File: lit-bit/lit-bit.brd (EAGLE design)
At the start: 37.5 x 43.8 mm, 71 parts, among them J2 USB_MICRO_B_SMD_FEMALE, J3 ISP, U2 32U4, U3 73831, U4 ADXL345, U5 S-1335, U6 MCP7940N, U7 24FC1025, Y1 8MHz, Y2 32.768kHz, Y3 32.768kHz, Y4 16MHz

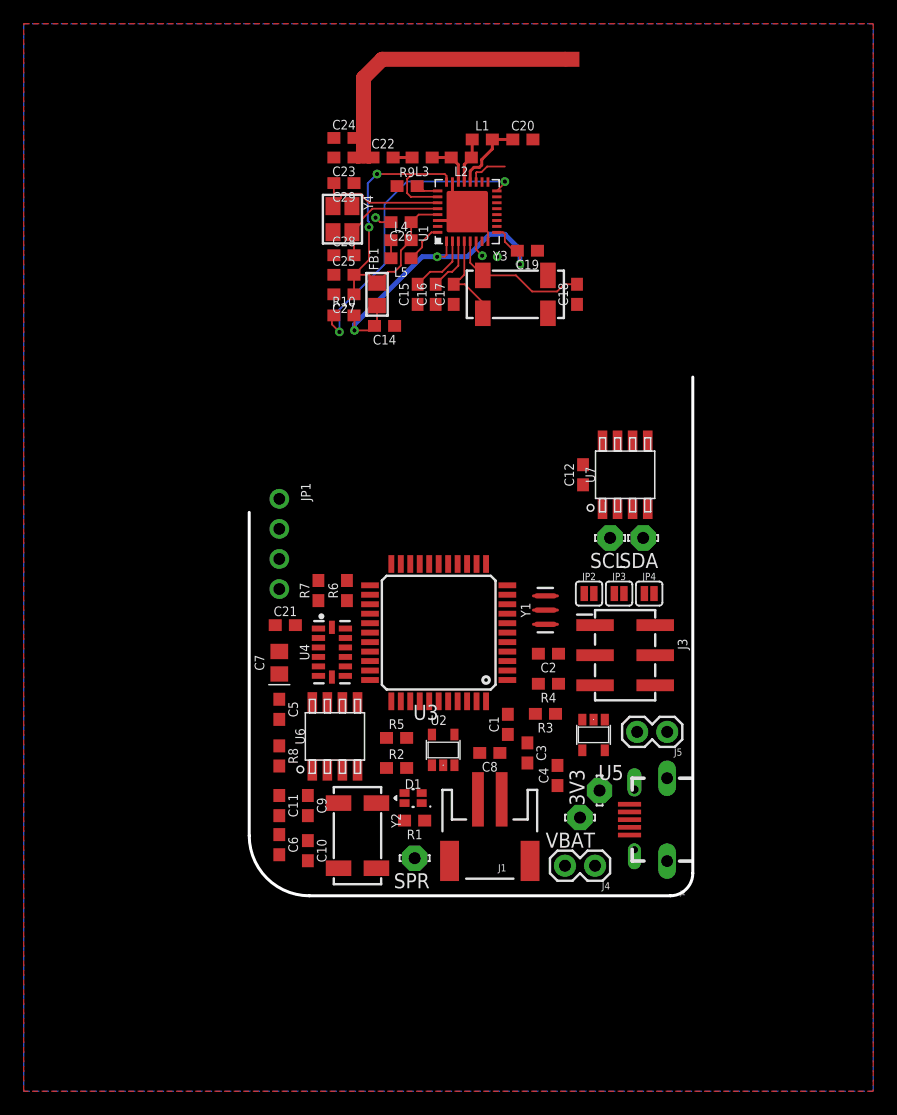
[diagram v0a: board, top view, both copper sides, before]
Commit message: fukky routed, but is ugly
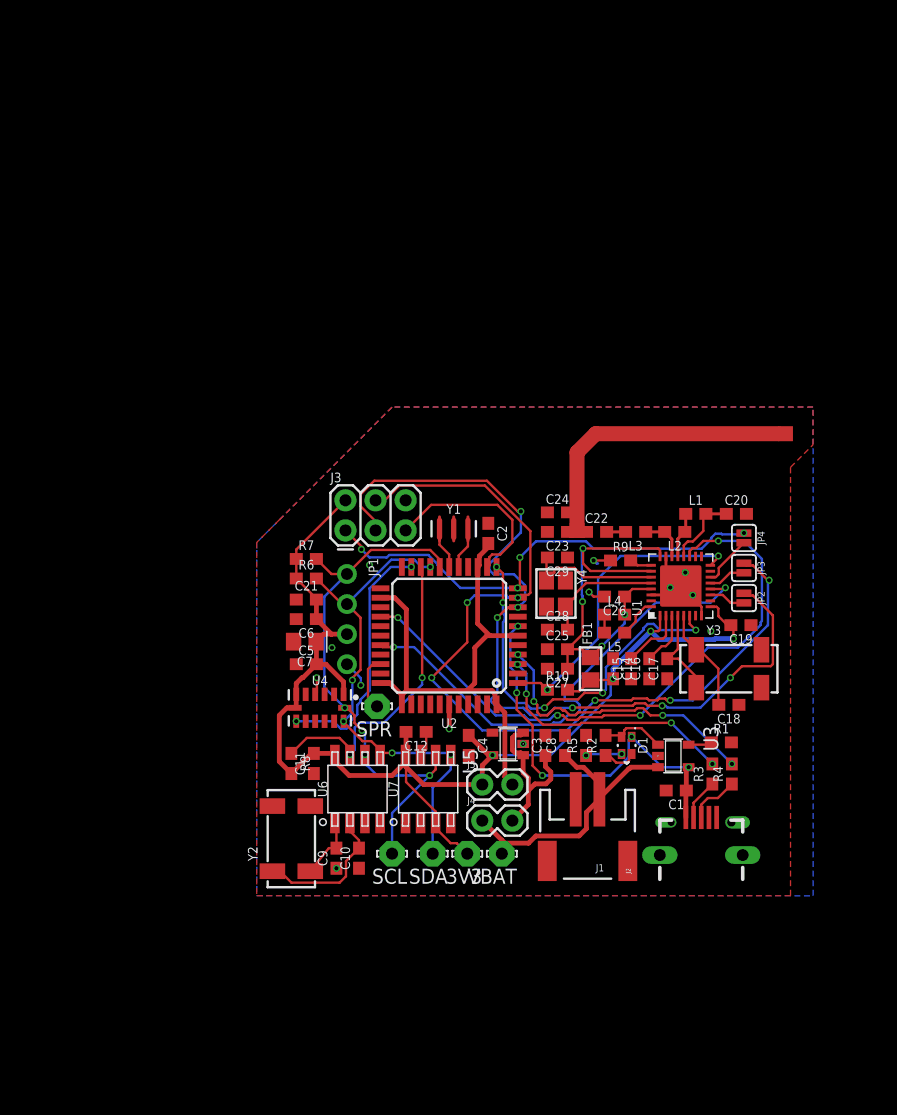
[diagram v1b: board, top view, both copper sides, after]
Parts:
- J3: device SCADA_CUSTOM_LIBRARY:2X3_SMD_HAND_SOLDER -> SCADA_CUSTOM_LIBRARY:2X3
- moved C18 37.0 mm to (39.9, 16.1), turned to 180 degrees
- moved C15 36.4 mm to (31.6, 19.2)
- moved C16 36.4 mm to (33.1, 19.2)
- moved C17 36.4 mm to (34.7, 19.2)
- moved C19 36.4 mm to (40.9, 22.9)
- moved C20 36.4 mm to (40.5, 32.3)
- moved C22 36.4 mm to (28.7, 30.7)
- moved C23 36.4 mm to (25.4, 30.7)
- moved C24 36.4 mm to (25.4, 32.4)
- moved C25 36.4 mm to (25.4, 20.8)
- moved C26 36.4 mm to (30.2, 25.3)
- moved C27 36.4 mm to (25.4, 19.2)
- moved C28 36.4 mm to (25.4, 22.5)
- moved C29 36.4 mm to (25.4, 28.6)
- moved FB1 36.4 mm to (28.2, 19.2)
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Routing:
- net 3V3: track 30.4 -> 110.1 mm, vias 3 -> 4
- net MOSI: track 0.00 -> 74.8 mm, vias 0 -> 6
- net SCK: track 0.00 -> 73.6 mm, vias 0 -> 6
- net NRF-RST: track 3.43 -> 52.5 mm, vias 0 -> 4
- net SCL: track 0.00 -> 46.8 mm, vias 0 -> 4
- net ITSYPWR: track 0.00 -> 45.7 mm
- net SDA: track 0.00 -> 43.0 mm, vias 0 -> 5
- net REQN: track 0.00 -> 41.2 mm, vias 0 -> 2
- net MISO: track 0.00 -> 40.1 mm, vias 0 -> 4
- net VUSB: track 0.00 -> 34.0 mm, vias 0 -> 5
- net ACTIVE: track 1.44 -> 33.4 mm, vias 1 -> 5
- net RTC-INT: track 0.00 -> 26.0 mm, vias 0 -> 2
- net VBAT: track 0.00 -> 25.4 mm
- net D+: track 0.00 -> 24.8 mm, vias 0 -> 4
- net N$6: track 0.00 -> 21.8 mm, vias 0 -> 4
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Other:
- board outline removed
